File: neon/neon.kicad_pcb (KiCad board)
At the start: 2 copper layers, 54.7 x 55 mm, 27 parts, among them J1 V3V3-VIO, J2 V3V3-GND, J3 V3V3-GND, J4 V3V3-GND, J5 VBUS-VCC, U1 FT4232H_module, U2 A, U3 B, U4 C, U5 D, U6 74HC595

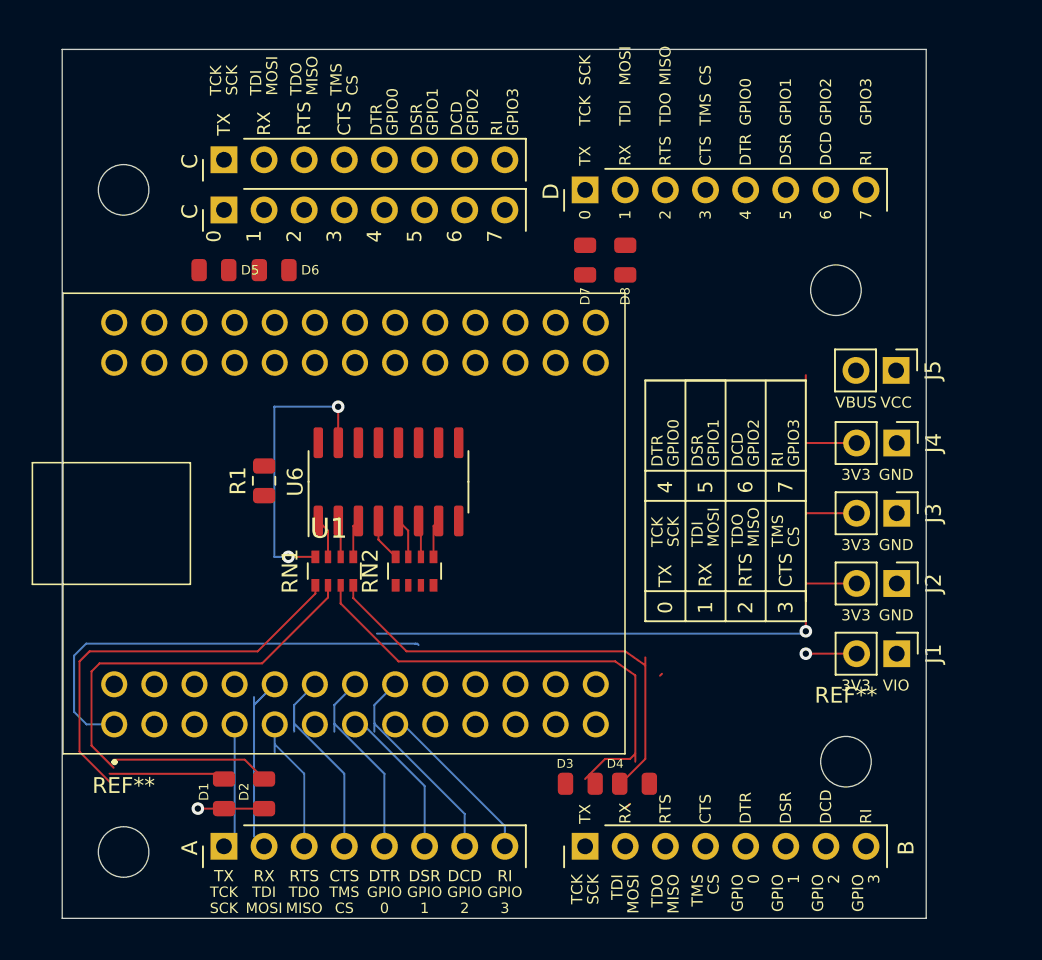
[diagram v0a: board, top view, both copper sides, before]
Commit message: With table and LEDs underneath the ftdi
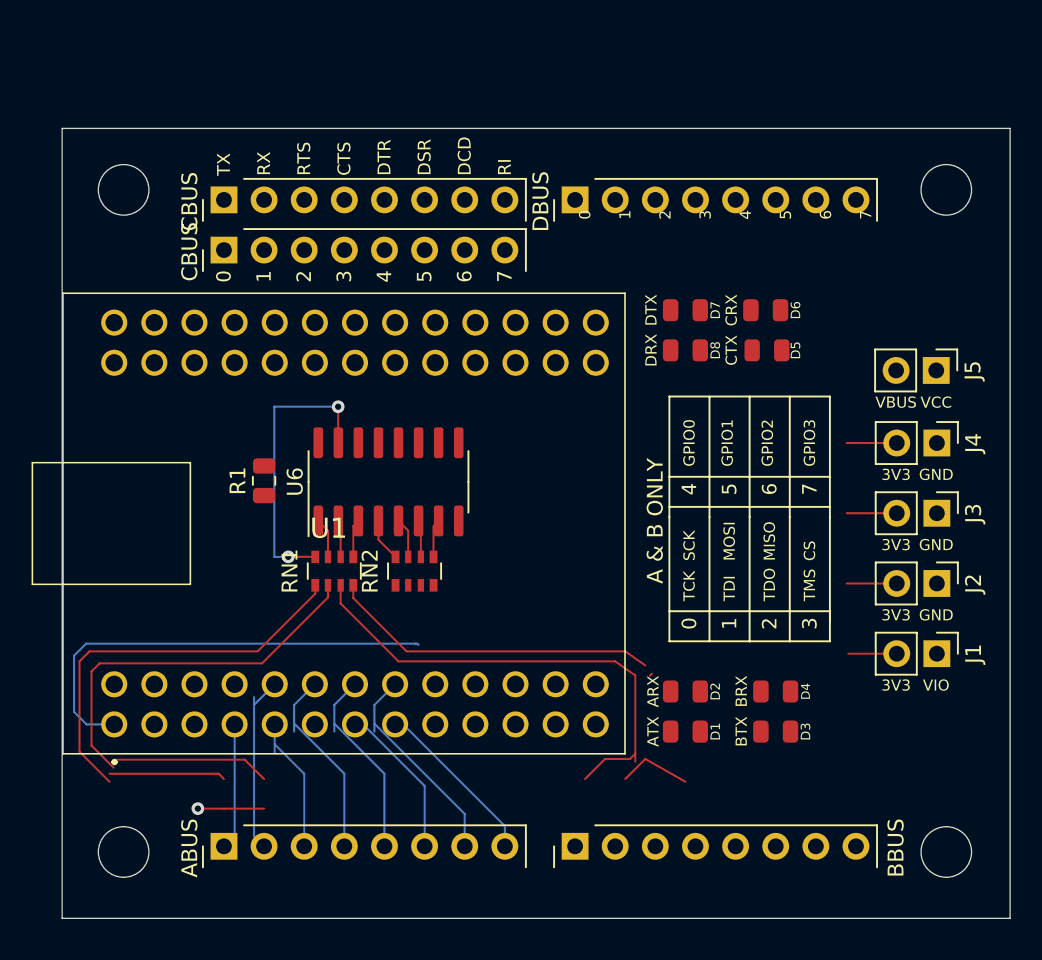
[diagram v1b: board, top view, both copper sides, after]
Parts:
- U2: value A -> ABUS
- U3: value B -> BBUS
- U4 (x2): value C -> CBUS
- U5: value D -> DBUS
- moved D5 35.4 mm to (160.1, 94.0)
- moved D6 31.2 mm to (160.0, 91.4)
- moved D1 29.5 mm to (154.9, 118.1), turned to 180 degrees
- moved D2 27.4 mm to (154.9, 115.6), turned to 180 degrees
- moved D3 12.8 mm to (160.7, 118.1), turned to 0 degrees
- moved D4 10.7 mm to (160.7, 115.6)
- moved REF** 9.44 mm to (171.4, 83.8)
- moved REF** 8.54 mm to (171.4, 125.7)
- moved D7 7.10 mm to (154.9, 91.4), turned to 180 degrees
- moved D8 6.87 mm to (154.9, 94.0), turned to 180 degrees
- moved J1 2.54 mm to (170.9, 113.2)
- moved J2 2.54 mm to (170.9, 108.7)
- moved J3 2.54 mm to (170.9, 104.3)
- moved J4 2.54 mm to (170.9, 99.8)
- moved J5 2.54 mm to (170.8, 95.2)
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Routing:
- net V3V3: track 84.6 -> 41.2 mm, vias 2 -> 0
- net GND: track 12.4 -> 4.19 mm
- net Net-(D4-Pad2): track 21.4 -> 25.7 mm
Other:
- board size 54.7 x 55 mm -> 60 x 50 mm
- board text added: "A & B ONLY"
- board text added: "ARX"
- board text added: "ATX"
- board text added: "BRX"
- board text added: "BTX"
- board text added: "CRX"
- board text added: "CTX"
- board text added: "DRX"
- board text added: "DTX"
- board text removed: "GPIO"
